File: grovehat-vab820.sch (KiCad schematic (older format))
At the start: 5 parts, among them P1 CONN_10X2, P2 CONN_4, P3 CONN_4, P4 CONN_4, P5 CONN_4

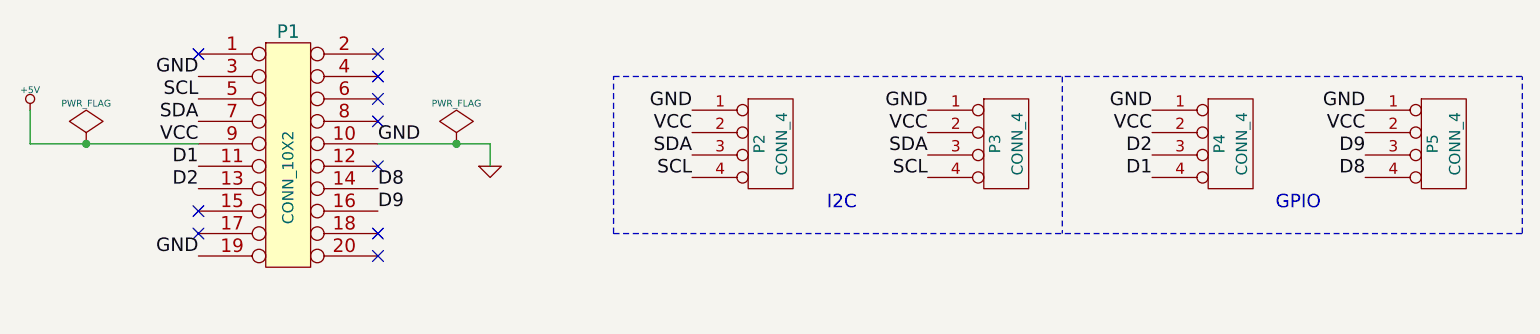
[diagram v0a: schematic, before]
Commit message: first draft of GrooveHat
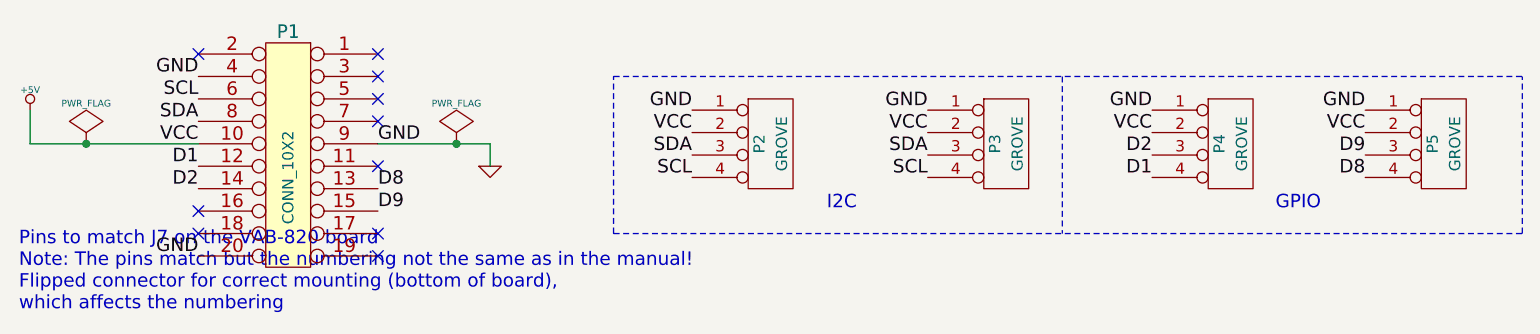
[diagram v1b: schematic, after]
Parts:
- P2, P3, P4, P5: value CONN_4 -> GROVE
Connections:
- net +5V: now also P1.10 (P10); no longer P1.9 (P9)
- net D1: now also P1.12 (P12); no longer P1.11 (P11)
- net D2: now also P1.14 (P14); no longer P1.13 (P13)
- net D8: now also P1.13 (P13); no longer P1.14 (P14)
- net D9: now also P1.15 (P15); no longer P1.16 (P16)
- net GND: now also P1.20 (P20), P1.4 (P4), P1.9 (P9); no longer P1.10 (P10), P1.19 (P19), P1.3 (P3)
- net SCL: now also P1.6 (P6); no longer P1.5 (P5)
- net SDA: now also P1.8 (P8); no longer P1.7 (P7)
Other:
- note added: "Pins to match J7 on the VAB-820 board\nNote: The pins match but the numbering not the same as in the manual!\nFlipped connector for correct mounting (bottom of board),\nwhich affects the numbering"
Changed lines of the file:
@@
 Sheet 1 1
 Title "GroveHat for VIA VAB-820"
-Date "13 aug 2015"
+Date "15 aug 2015"
 Rev "1"
 Comp "Moonpunch"
@@
 F 7 "http://www.mouser.tw/ProductDetail/3M-Electronic-Solutions-Division/950420-6102-AR/" H 3250 3750 60  0001 C CNN "S1L"
 	1    3250 3750
-	1    0    0    -1
+	-1   0    0    -1
 $EndComp
 $Comp
@@
 P 5400 3700
 F 0 "P2" V 5350 3700 50  0000 C CNN
-F 1 "CONN_4" V 5450 3700 50  0000 C CNN
+F 1 "GROVE" V 5450 3700 50  0000 C CNN
 F 2 "TWIG_2.0" H 5400 3700 60  0001 C CNN
 F 3 "http://www.seeedstudio.com/depot/images/opl/datasheet/3470130P1.pdf" H 5400 3700 60  0001 C CNN
@@
 P 6450 3700
 F 0 "P3" V 6400 3700 50  0000 C CNN
-F 1 "CONN_4" V 6500 3700 50  0000 C CNN
+F 1 "GROVE" V 6500 3700 50  0000 C CNN
 F 2 "TWIG_2.0" H 5400 3700 60  0001 C CNN
 F 3 "http://www.seeedstudio.com/depot/images/opl/datasheet/3470130P1.pdf" H 5400 3700 60  0001 C CNN
@@
 P 7450 3700
 F 0 "P4" V 7400 3700 50  0000 C CNN
-F 1 "CONN_4" V 7500 3700 50  0000 C CNN
+F 1 "GROVE" V 7500 3700 50  0000 C CNN
 F 2 "TWIG_2.0" H 5400 3700 60  0001 C CNN
 F 3 "http://www.seeedstudio.com/depot/images/opl/datasheet/3470130P1.pdf" H 5400 3700 60  0001 C CNN
@@
 P 8400 3700
 F 0 "P5" V 8350 3700 50  0000 C CNN
-F 1 "CONN_4" V 8450 3700 50  0000 C CNN
+F 1 "GROVE" V 8450 3700 50  0000 C CNN
 F 2 "TWIG_2.0" H 5400 3700 60  0001 C CNN
 F 3 "http://www.seeedstudio.com/depot/images/opl/datasheet/3470130P1.pdf" H 5400 3700 60  0001 C CNN
@@
 	2100 3700 2850 3700
 Connection ~ 2350 3700
+Text Notes 2050 4450 0    60   ~ 0
+Pins to match J7 on the VAB-820 board\nNote: The pins match but the numbering not the same as in the manual!\nFlipped connector for correct mounting (bottom of board),\nwhich affects the numbering
 $EndSCHEMATC
